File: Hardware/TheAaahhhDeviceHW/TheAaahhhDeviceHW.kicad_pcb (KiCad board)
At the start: 2 copper layers, 13 parts, among them J1 Speaker, J2 WS_LEDStrip, J3 WeMos_D1_Breakout, J4 DFPlayerMini_Breakout, U1 WeMos_D1_mini, U2 DFPlayerMini

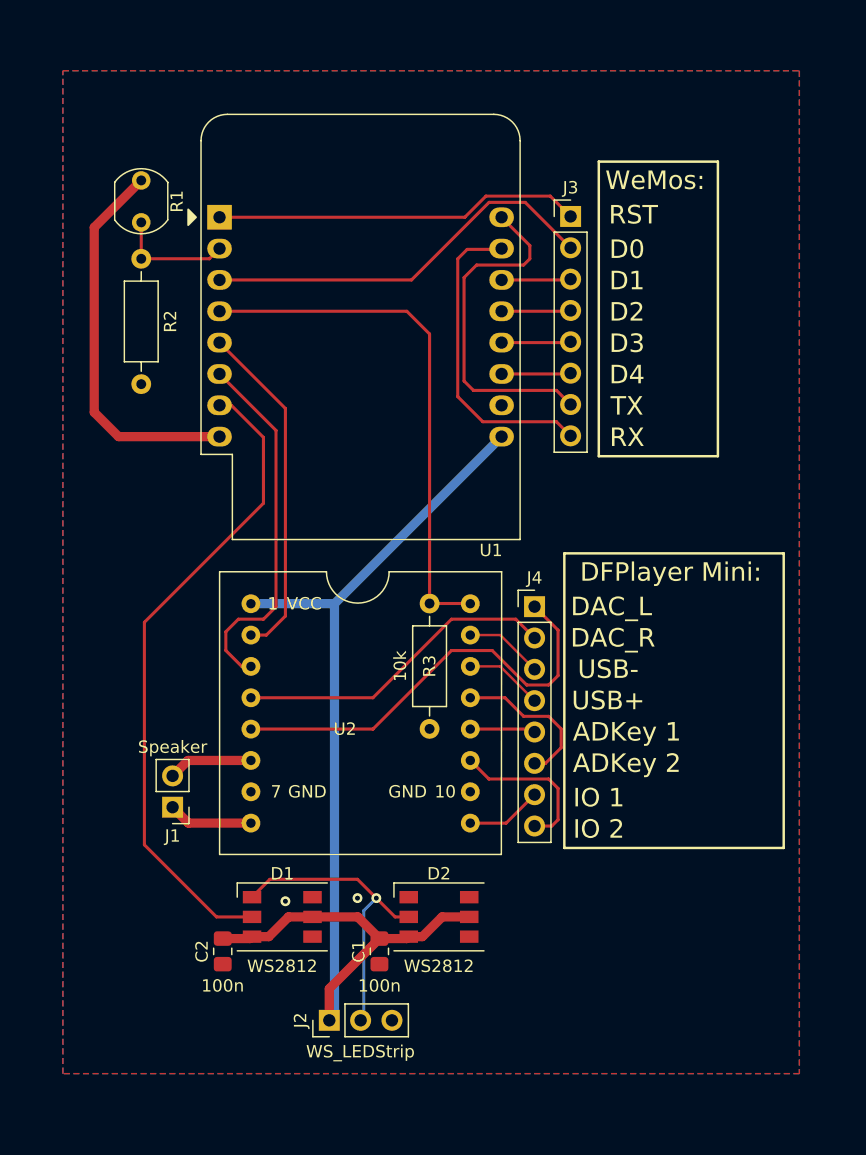
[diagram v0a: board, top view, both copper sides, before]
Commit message: v1
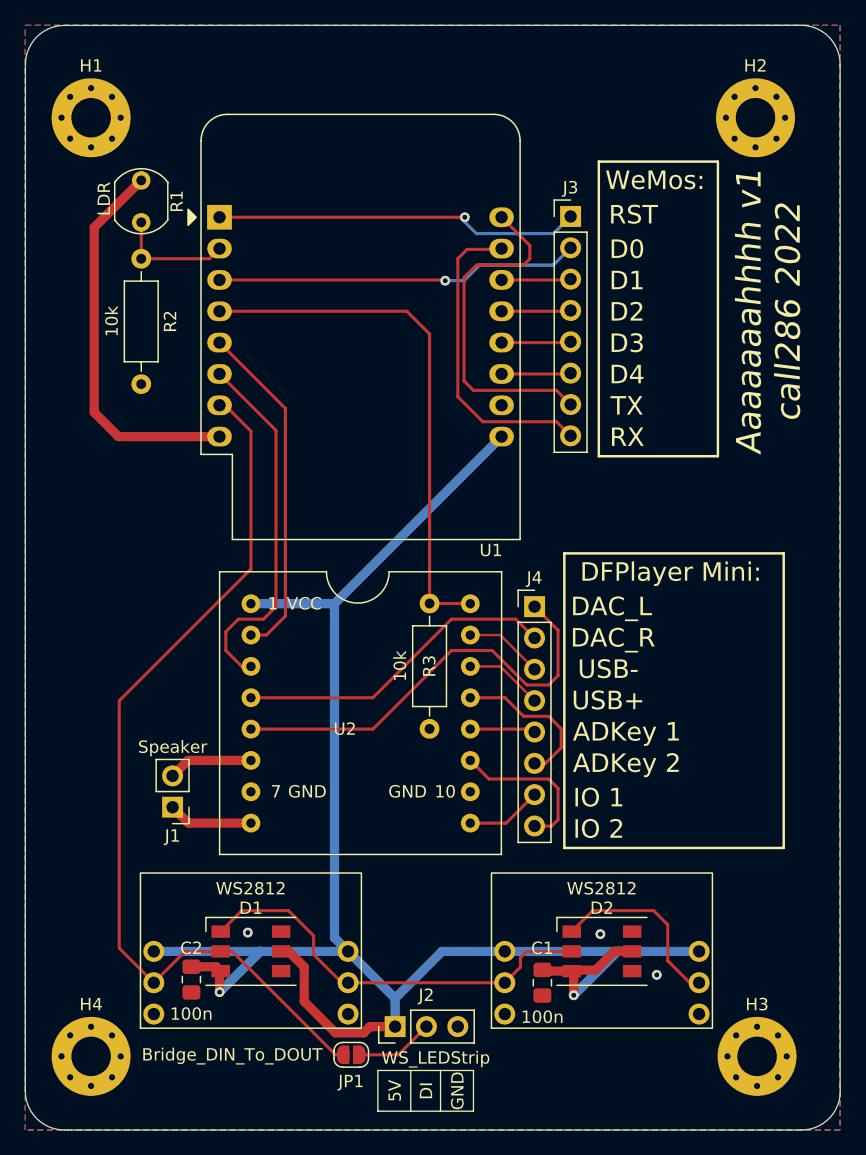
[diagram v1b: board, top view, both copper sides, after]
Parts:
- added H1: MountingHole, MountingHole:MountingHole_3.2mm_M3_Pad_Via, F.Cu at (109.0, 85.1)
- added H2: MountingHole, MountingHole:MountingHole_3.2mm_M3_Pad_Via, F.Cu at (162.8, 85.1)
- added H3: MountingHole, MountingHole:MountingHole_3.2mm_M3_Pad_Via, F.Cu at (162.9, 161.2)
- added H4: MountingHole, MountingHole:MountingHole_3.2mm_M3_Pad_Via, F.Cu at (109.0, 161.2)
- added JP1: Bridge_DIN_To_DOUT, Jumper:SolderJumper-2_P1.3mm_Open_RoundedPad1.0x1.5mm, F.Cu at (130.0, 161.0)
- D1, D2: footprint LED_SMD:LED_WS2812_PLCC6_5.0x5.0mm_P1.6mm -> DCDModules:LED_WS2812+SMD
- moved D2 13.5 mm to (150.4, 152.7)
- moved C1 13.5 mm to (145.5, 155.2)
- moved J2 5.36 mm to (133.6, 158.8)
- moved D1 3.78 mm to (121.9, 152.7)
- moved C2 3.42 mm to (117.1, 154.9)
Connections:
- J2 pad 2: WS_DOut -> WS_DInOut
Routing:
- net +5V: track 90.3 -> 142.2 mm, vias 0 -> 2
- net WS_DIn: track 52.8 -> 73.7 mm
- net unconnected-(D2-Pad1): track 0.00 -> 15.2 mm
- net WS_DOut: track 25.0 -> 34.0 mm, vias 1 -> 0
- net WS_DInOut: track 0.00 -> 6.39 mm
- net D0: track 32.6 -> 29.6 mm, vias 0 -> 1
- net RST: vias 0 -> 1
- net GND: vias 2 -> 3
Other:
- board outline added: 66.1 x 89.5 mm
- board text added: "5V"
- board text added: "Aaaaaaahhhh v1"
- board text added: "DI"
- board text added: "GND"
- board text added: "call286 2022"
